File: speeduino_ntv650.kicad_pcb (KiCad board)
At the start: 2 copper layers, 75 x 120 mm, 76 parts, among them IC1 SP721, IC2 TC4424, J1 DB25_Male_MountingHoles, J2 Conn_01x01, J3 Conn_01x01, J4 Conn_01x01, J5 Conn_01x01, P1 MAX9926_9927, Q1 STP62NS04Z, Q2 STP62NS04Z, Q3 STP62NS04Z, U1 LM2937xT

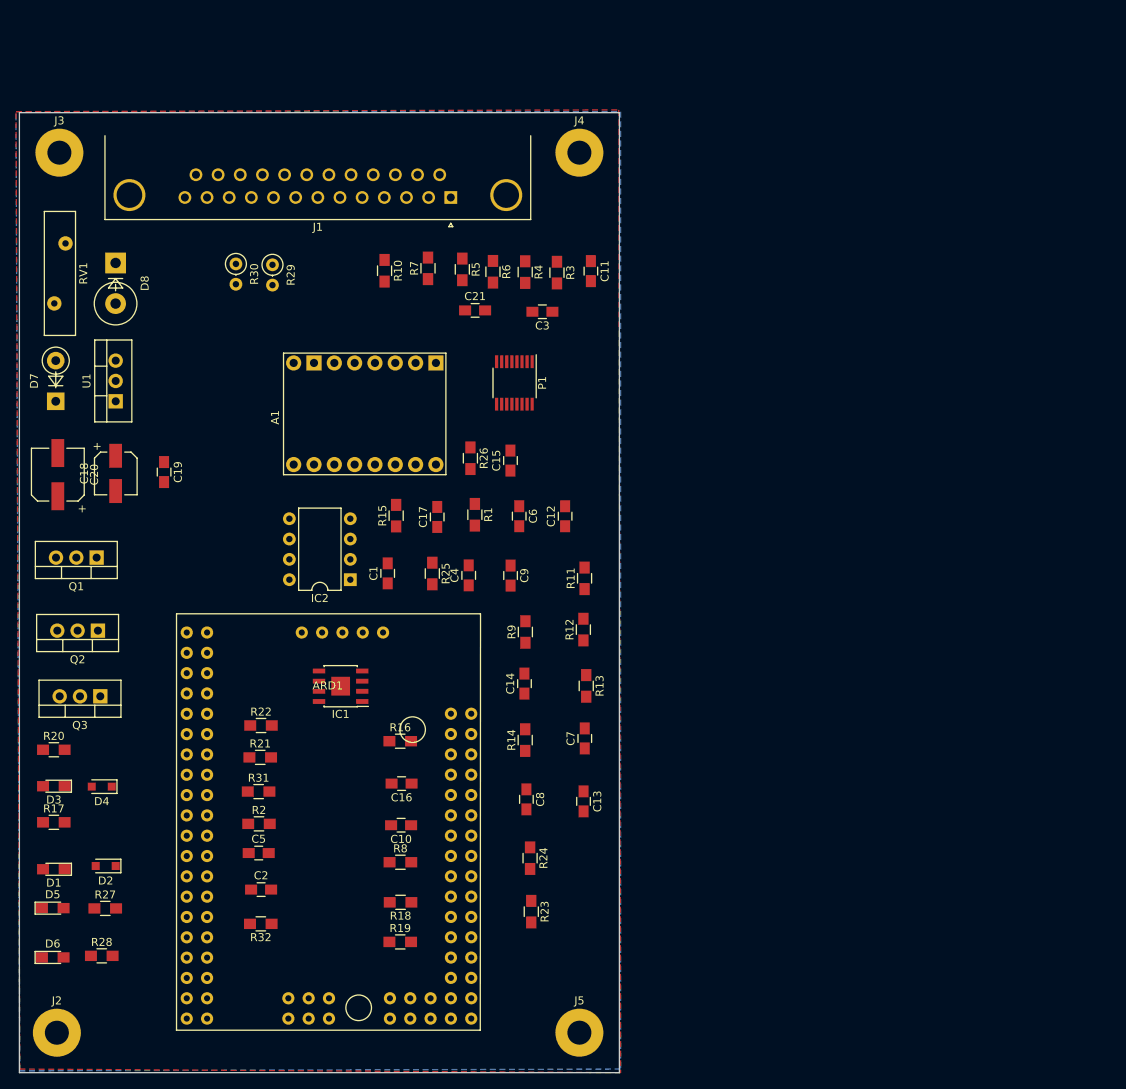
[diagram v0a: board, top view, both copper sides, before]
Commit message: pcb frame complited
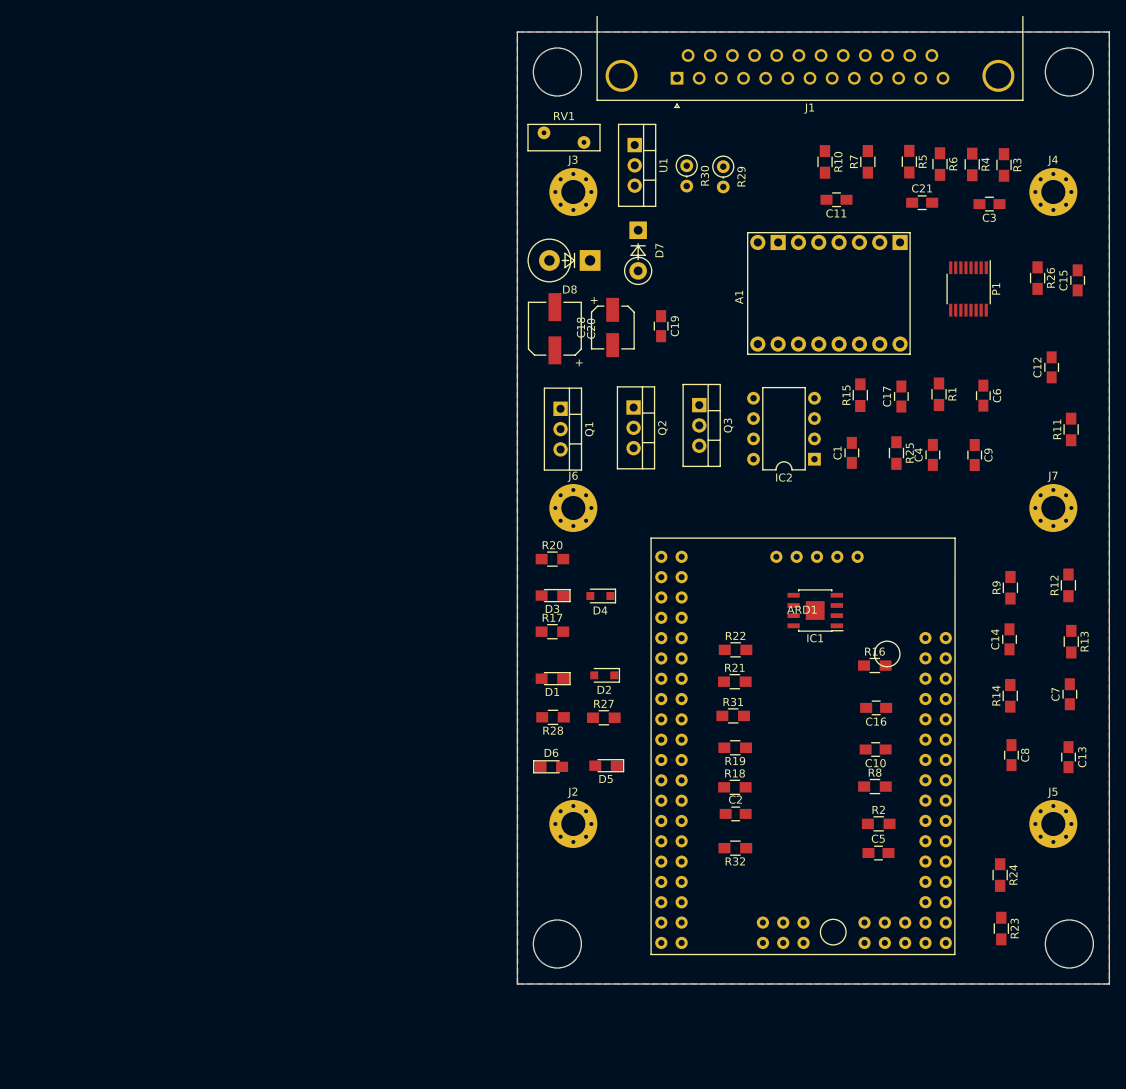
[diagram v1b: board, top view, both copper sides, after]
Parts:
- added J6: Conn_01x01, Mounting_Holes:MountingHole_3mm_Pad_Via, F.Cu at (119.1, 100.5)
- added J7: Conn_01x01, Mounting_Holes:MountingHole_3mm_Pad_Via, F.Cu at (179.1, 100.5)
- J1: value DB25_Male_MountingHoles -> DB25_Female_MountingHoles; footprint Connector_Dsub:DSUB-25_Male_Horizontal_P2.77x2.84mm_EdgePinOffset4.94mm_Housed_MountingHolesOffset7.48mm -> ntv650_ecu:DSUB-25_Female_Horizontal_P2.77x2.84mm_EdgePinOffset4.94mm_Housed_MountingHolesOffset7.48mm
- J2, J3, J4, J5: footprint MountingHole:MountingHole_3mm_Pad -> Mounting_Holes:MountingHole_3mm_Pad_Via
- RV1: footprint Varistors:RV_Disc_D15.5_W3.9_P7.5 -> Varistors:RV_Disc_D9_W3.3_P5
- moved Q3 83.2 mm to (134.8, 87.7), turned to 270 degrees
- moved C5 77.5 mm to (157.2, 143.7)
- moved R2 77.5 mm to (157.2, 140.0)
- moved D7 75.9 mm to (127.2, 65.8), turned to 270 degrees
- moved C15 74.4 mm to (182.1, 72.1)
- moved R26 74.4 mm to (177.1, 71.8)
- moved Q2 72.5 mm to (126.6, 88.0), turned to 270 degrees
- moved U1 72.4 mm to (126.7, 55.2), turned to 270 degrees
- moved D5 71.4 mm to (123.2, 132.8), turned to 180 degrees
- moved J2 69.6 mm to (119.1, 140.0)
- moved RV1 69.2 mm to (120.4, 54.8), turned to 180 degrees
- moved D2 66.7 mm to (122.9, 121.5)
- moved D3 66.7 mm to (116.5, 111.5)
- moved D4 66.7 mm to (122.4, 111.5)
- moved D6 66.7 mm to (116.3, 132.9)
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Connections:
- J1 pad 1: VR1+ -> GND
- J1 pad 10: ign-1-out -> 5V
- J1 pad 11: idle-out -> MAP
- J1 pad 12: 12V -> VR2+
- J1 pad 13: GND -> VR1+
- J1 pad 14: VR1- -> GND
- J1 pad 15: VR2- -> 12V
- J1 pad 16: GND -> ign-2-out
- J1 pad 17: GND -> inj-2-out
- J1 pad 18: TPS_sens -> STEP-2B-OUT
- J1 pad 19: ITS_sens -> STEP-1B-OUT
- J1 pad 2: VR2+ -> 12V
- J1 pad 20: STEP-1B-OUT -> ITS_sens
- J1 pad 21: STEP-2B-OUT -> TPS_sens
- J1 pad 22: inj-2-out -> GND
- J1 pad 23: ign-2-out -> GND
- J1 pad 24: 12V -> VR2-
- J1 pad 25: GND -> VR1-
- J1 pad 3: MAP -> idle-out
- J1 pad 4: 5V -> ign-1-out
- J1 pad 5: O2_sens -> inj-1-out
- J1 pad 6: CLT_sens -> STEP-2A-OUT
- J1 pad 8: STEP-2A-OUT -> CLT_sens
- J1 pad 9: inj-1-out -> O2_sens
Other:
- board size 75 x 120 mm -> 74 x 119 mm
